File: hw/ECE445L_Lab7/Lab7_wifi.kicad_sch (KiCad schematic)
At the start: 4 parts, among them U1 ESP8266-1

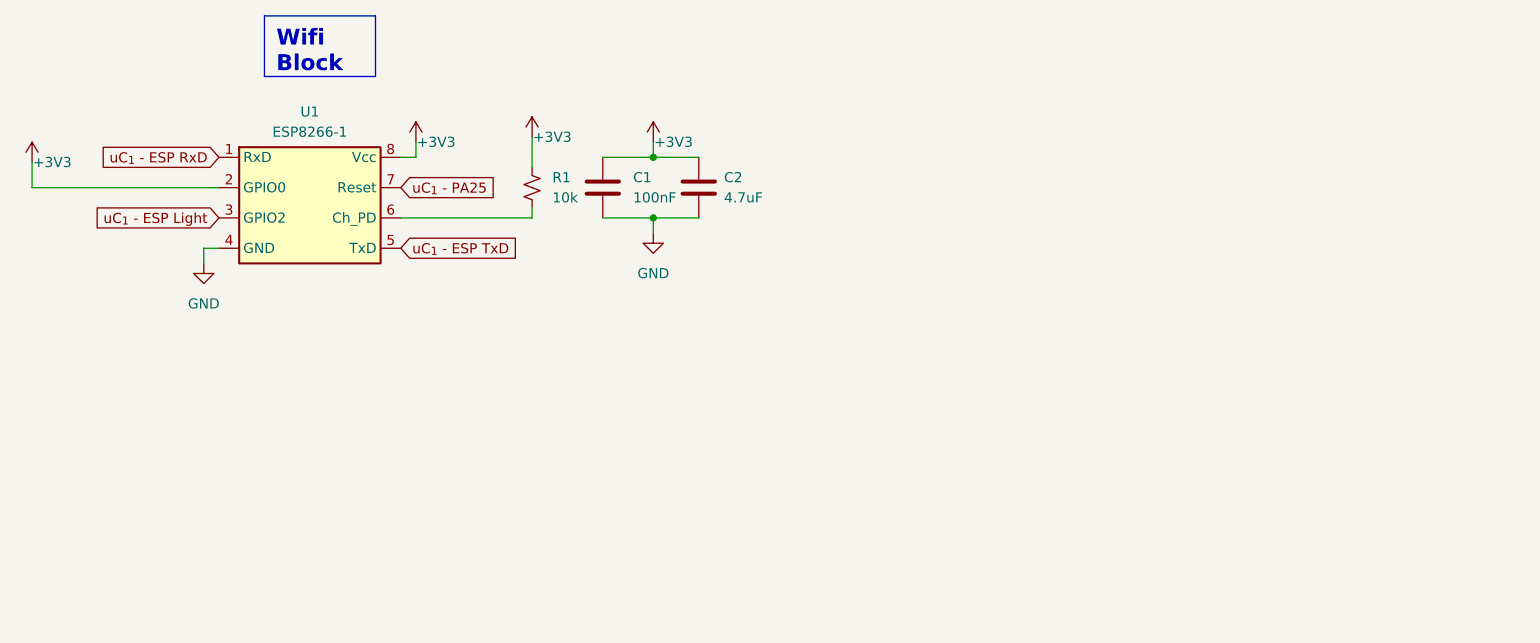
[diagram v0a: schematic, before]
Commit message: almost finished with schem
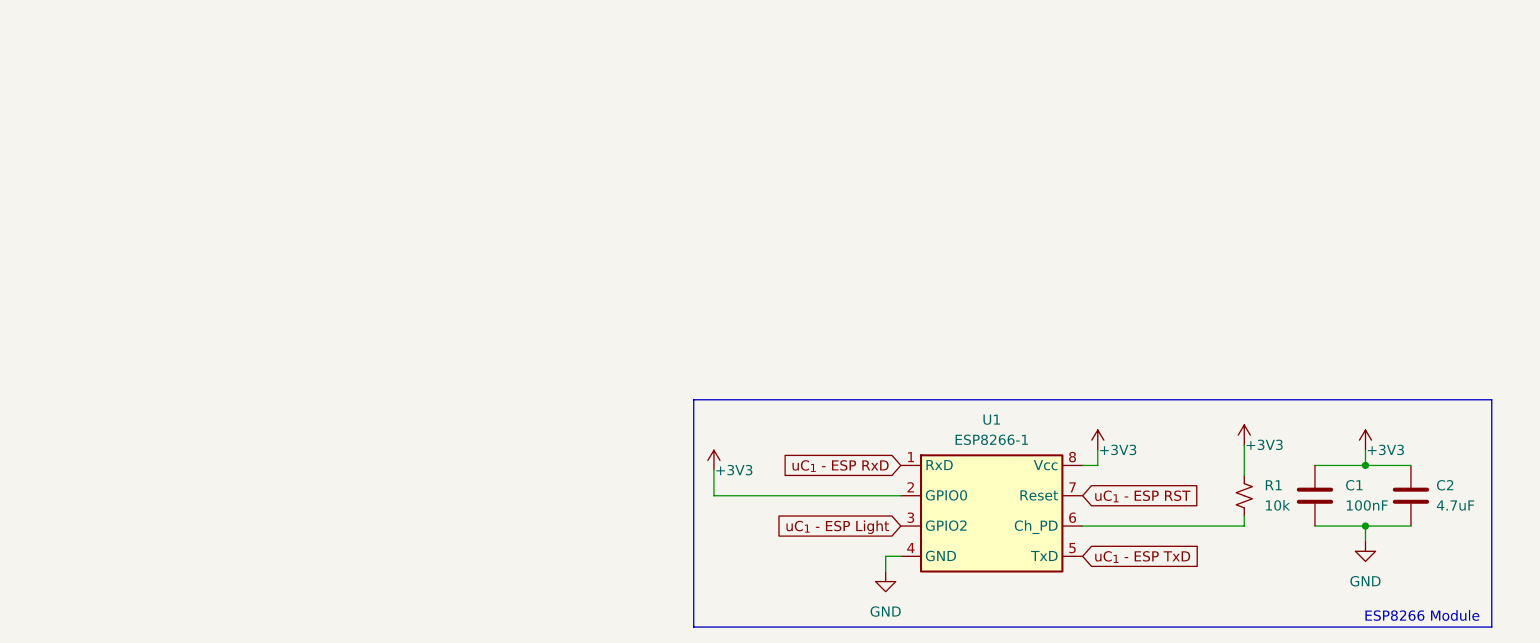
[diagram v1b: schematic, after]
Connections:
- net uC_{1} - PA25 renamed uC_{1} - ESP RST
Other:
- note added: "ESP8266 Module"
- moved on the sheet: C1, C2, R1, U1

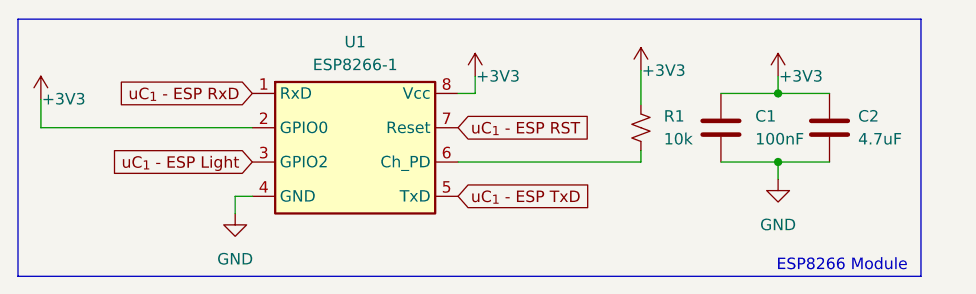
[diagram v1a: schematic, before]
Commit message: finished prelim schem
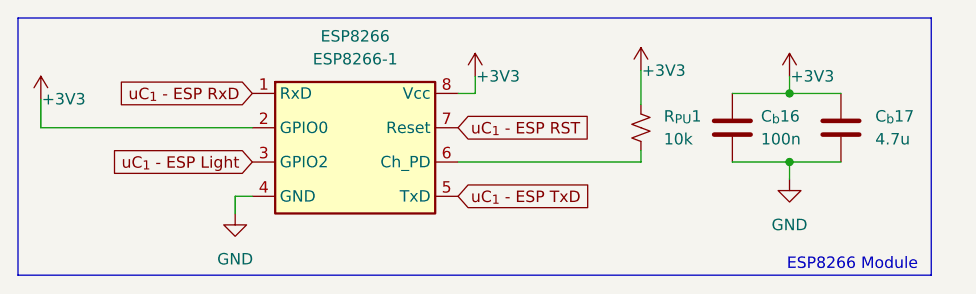
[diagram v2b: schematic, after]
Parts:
- C_{b}16: renamed from C1; value 100nF -> 100n; footprint ECE445L:C_Radial_100mil -> Capacitor_SMD:C_0603_1608Metric_Pad1.08x0.95mm_HandSolder; Distributor (none) -> Mouser; Manufacturer (none) -> Walsin; Manufacturer_Part_Number (none) -> 0603B104J160CT; Mouser Part Number (none) -> 791-0603B104J160CT
- C_{b}17: renamed from C2; value 4.7uF -> 4.7u; footprint ECE445L:CP_Radial_Tantal200mil -> Capacitor_SMD:C_0603_1608Metric_Pad1.08x0.95mm_HandSolder; Distributor (none) -> Mouser; Manufacturer (none) -> Walsin; Manufacturer_Part_Number (none) -> 0805X475M250CT; Mouser Part Number (none) -> 791-0805X475M250CT
- ESP8266: renamed from U1; Distributor (none) -> 445L
- R_{PU}1: renamed from R1; footprint ECE445L:R_Axial_DIN0204_L3.6mm_D1.6mm_P7.62mm_Horizontal -> Resistor_SMD:R_0805_2012Metric_Pad1.20x1.40mm_HandSolder; Distributor (none) -> Mouser; Manufacturer (none) -> Bourns; Manufacturer_Part_Number (none) -> CRM0805-FX-1002ELF; Mouser Part Number (none) -> 652-CRM0805FX1002ELF
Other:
- moved on the sheet: C_{b}16, C_{b}17

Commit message: handoff to jonathan until midnight
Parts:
- C_{b}17, R_{PU}1: Distributor Mouser -> Valvano
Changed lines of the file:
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@@
 			)
 		)
-		(property "Distributor" "Mouser"
+		(property "Distributor" "Valvano"
 			(at 194.31 96.52 0)
 			(hide yes)
@@
 			)
 		)
-		(property "Distributor" "Mouser"
+		(property "Distributor" "Valvano"
 			(at 172.085 96.52 0)
 			(hide yes)
